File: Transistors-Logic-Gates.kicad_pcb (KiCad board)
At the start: 2 copper layers, 92.5 x 115.5 mm, 31 parts, among them J1 Conn_01x05_Socket, Q1 PN2222A, Q2 PN2222A, Q3 PN2222A, Q4 PN2222A, Q5 PN2222A, Q6 PN2222A, Q7 PN2222A, SW1 SW_SPDT, SW2 SW_SPDT, SW3 SW_SPDT, SW4 SW_SPDT, SW5 SW_Push, SW6 SW_SPDT, SW7 SW_SPDT

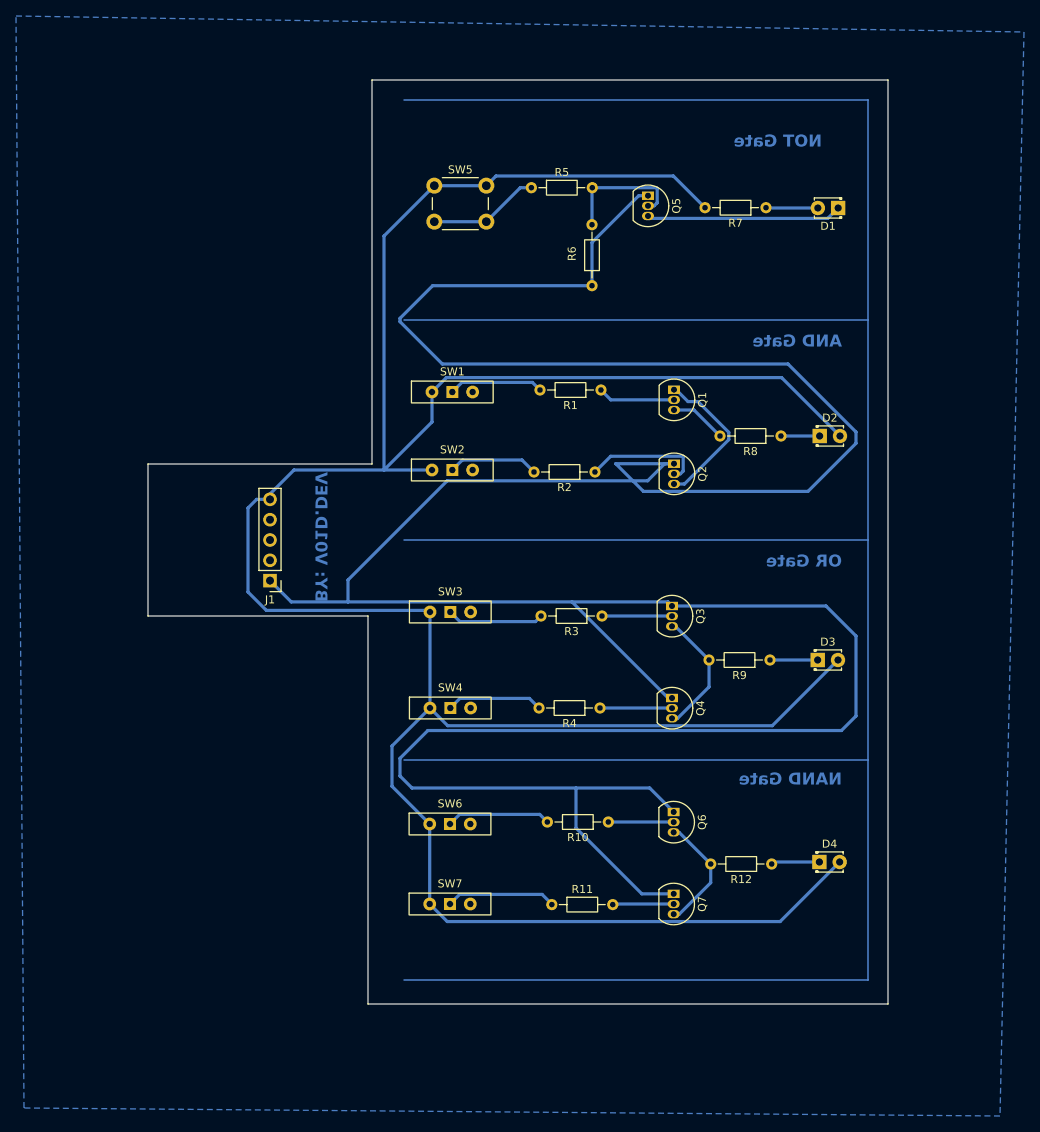
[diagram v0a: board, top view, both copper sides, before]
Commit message: feat: first PCB made, still issue to iron out
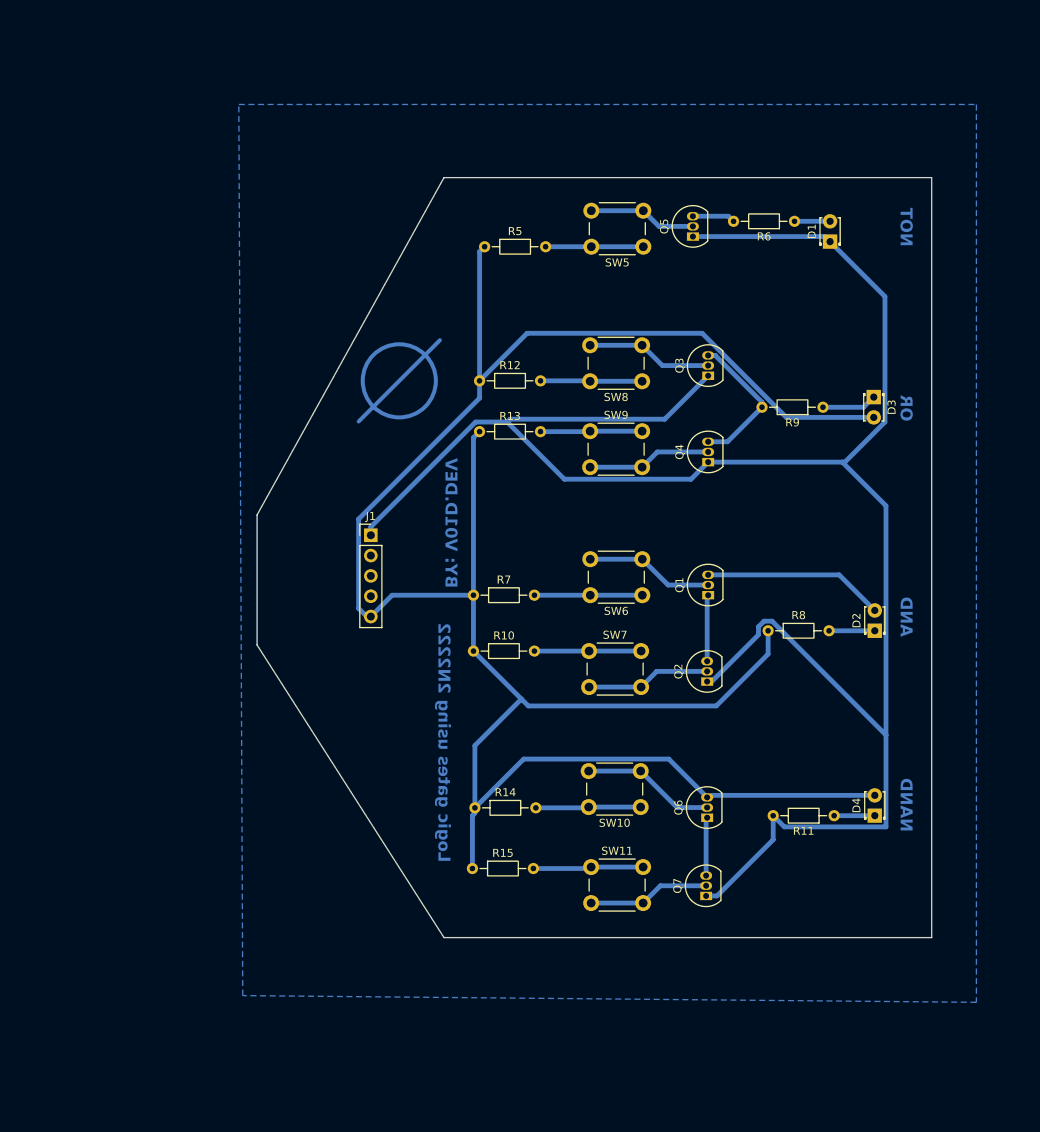
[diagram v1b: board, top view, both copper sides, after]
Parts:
- removed R1, R2, R3, R4: 4.7K, Resistor_THT:R_Axial_DIN0204_L3.6mm_D1.6mm_P7.62mm_Horizontal
- removed SW1, SW2, SW3, SW4: SW_SPDT, Button_Switch_THT:SW_Slide-03_Wuerth-WS-SLTV_10x2.5x6.4_P2.54mm
- added R13: 10K, Resistor_THT:R_Axial_DIN0204_L3.6mm_D1.6mm_P7.62mm_Horizontal, F.Cu at (131.4, 76.5)
- added R14: 10K, Resistor_THT:R_Axial_DIN0204_L3.6mm_D1.6mm_P7.62mm_Horizontal, F.Cu at (130.9, 123.5)
- added R15: 10K, Resistor_THT:R_Axial_DIN0204_L3.6mm_D1.6mm_P7.62mm_Horizontal, F.Cu at (130.6, 131.1)
- added SW10: SW_Push, Button_Switch_THT:SW_PUSH_6mm_H5mm, F.Cu at (151.6, 123.4)
- added SW11: SW_Push, Button_Switch_THT:SW_PUSH_6mm_H5mm, F.Cu at (145.4, 130.9)
- added SW8: SW_Push, Button_Switch_THT:SW_PUSH_6mm_H5mm, F.Cu at (151.8, 70.2)
- added SW9: SW_Push, Button_Switch_THT:SW_PUSH_6mm_H5mm, F.Cu at (145.3, 76.4)
- R10: value 4.7K -> 10K
- R11: value 4.7K -> 470
- R12, R9: value 180 -> 10K
- R5: value 6.8K -> 10K
- R6: value 68K -> 1K
- R7: value 200 -> 10K
- R8: value 180 -> 1K
- SW6, SW7: value SW_SPDT -> SW_Push; footprint Button_Switch_THT:SW_Slide-03_Wuerth-WS-SLTV_10x2.5x6.4_P2.54mm -> Button_Switch_THT:SW_PUSH_6mm_H5mm
- moved R12 70.6 mm to (131.4, 70.1), turned to 0 degrees
- moved R7 60.7 mm to (130.7, 96.9), turned to 0 degrees
- moved SW6 37.4 mm to (151.8, 96.9), turned to 180 degrees
- moved R11 37.0 mm to (175.8, 124.5), turned to 180 degrees
- moved SW7 36.1 mm to (145.1, 103.9)
- moved D3 33.6 mm to (180.7, 72.1), turned to -90 degrees
- moved R9 32.3 mm to (174.4, 73.4)
- moved Q4 29.8 mm to (160.0, 80.3), turned to 90 degrees
- moved Q3 29.1 mm to (160.0, 69.5), turned to 90 degrees
- moved Q2 27.5 mm to (159.9, 107.7), turned to 90 degrees
- moved SW5 27.2 mm to (151.9, 53.3), turned to 180 degrees
- moved R10 27.2 mm to (130.7, 103.9), turned to 0 degrees
- moved R6 26.6 mm to (170.8, 50.2), turned to 180 degrees
- moved Q1 26.0 mm to (160.0, 96.9), turned to 90 degrees
- moved D2 25.3 mm to (180.8, 101.3), turned to 90 degrees
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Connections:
- D1 pad 1: Net-(D1-K) -> /GND
- D2 pad 2: /Vcc -> Net-(D2-A)
- Q1 pad 3: Net-(Q1-C) -> Net-(D2-A)
- Q5 pad 3: Net-(D1-K) -> Net-(Q5-C)
- Q6 pad 1: /GND -> Net-(Q6-E)
- Q6 pad 3: Net-(Q6-C) -> /Vcc
- Q7 pad 3: Net-(Q6-C) -> Net-(Q6-E)
- R10 pad 1: Net-(Q6-B) -> /Vcc
- R10 pad 2: Net-(SW6-A) -> Net-(R10-Pad2)
- R11 pad 1: Net-(Q7-B) -> Net-(D4-K)
- R11 pad 2: Net-(SW7-A) -> /GND
- R12 pad 1: Net-(D4-K) -> /Vcc
- R12 pad 2: Net-(Q6-C) -> Net-(R12-Pad2)
- R5 pad 1: Net-(R5-Pad1) -> /Vcc
- R5 pad 2: Net-(Q5-B) -> Net-(R5-Pad2)
- R6 pad 1: /GND -> Net-(D1-A)
- R6 pad 2: Net-(Q5-B) -> Net-(Q5-C)
- R7 pad 1: Net-(D1-A) -> /Vcc
- R7 pad 2: /Vcc -> Net-(R7-Pad2)
- R8 pad 1: Net-(D2-K) -> /Vcc
- R8 pad 2: Net-(Q1-C) -> Net-(D2-K)
- SW5 pad 1: /Vcc -> Net-(R5-Pad2)
- SW5 pad 2: Net-(R5-Pad1) -> Net-(Q5-B)
- SW6 pad 1: Net-(SW6-A) -> Net-(R7-Pad2)
- SW6 pad 2: /Vcc -> Net-(Q1-B)
- SW7 pad 1: Net-(SW7-A) -> Net-(R10-Pad2)
- SW7 pad 2: /Vcc -> Net-(Q2-B)
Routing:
- net /GND: track 417.5 -> 256.3 mm
- net /Vcc: track 351.8 -> 275.3 mm
- net Net-(D1-K): track 24.0 -> 0.00 mm
- net Net-(D2-A): track 0.00 -> 22.7 mm
- net Net-(Q6-C): track 14.9 -> 0.00 mm
- net Net-(R5-Pad1): track 13.9 -> 0.00 mm
- net Net-(R15-Pad2): track 0.00 -> 13.8 mm
- net Net-(SW7-A): track 13.7 -> 0.00 mm
- net Net-(R7-Pad2): track 0.00 -> 13.5 mm
- net Net-(R10-Pad2): track 0.00 -> 13.3 mm
- net Net-(R14-Pad2): track 0.00 -> 13.1 mm
- net Net-(SW6-A): track 13.1 -> 0.00 mm
- net Net-(R12-Pad2): track 0.00 -> 12.7 mm
- net Net-(R13-Pad2): track 0.00 -> 12.7 mm
- net Net-(R5-Pad2): track 0.00 -> 12.2 mm
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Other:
- board size 92.5 x 115.5 mm -> 84.3 x 95 mm
- board text added: "AND"
- board text added: "Logic gates using 2N2222"
- board text added: "NAND"
- board text added: "NOT"
- board text added: "OR"
- board text removed: "AND Gate"
- board text removed: "NAND Gate"
- board text removed: "NOT Gate"
- board text removed: "OR Gate"
